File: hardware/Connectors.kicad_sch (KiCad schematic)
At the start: 18 parts, among them J1 USB_C_Receptacle_USB2.0, J14 Conn_01x05, J2 M80-5302642, J3 M300-MV31045M1, J4 M80-5L10442MC, J5 M80-5L10442MC, J6 M80-5L10442MC

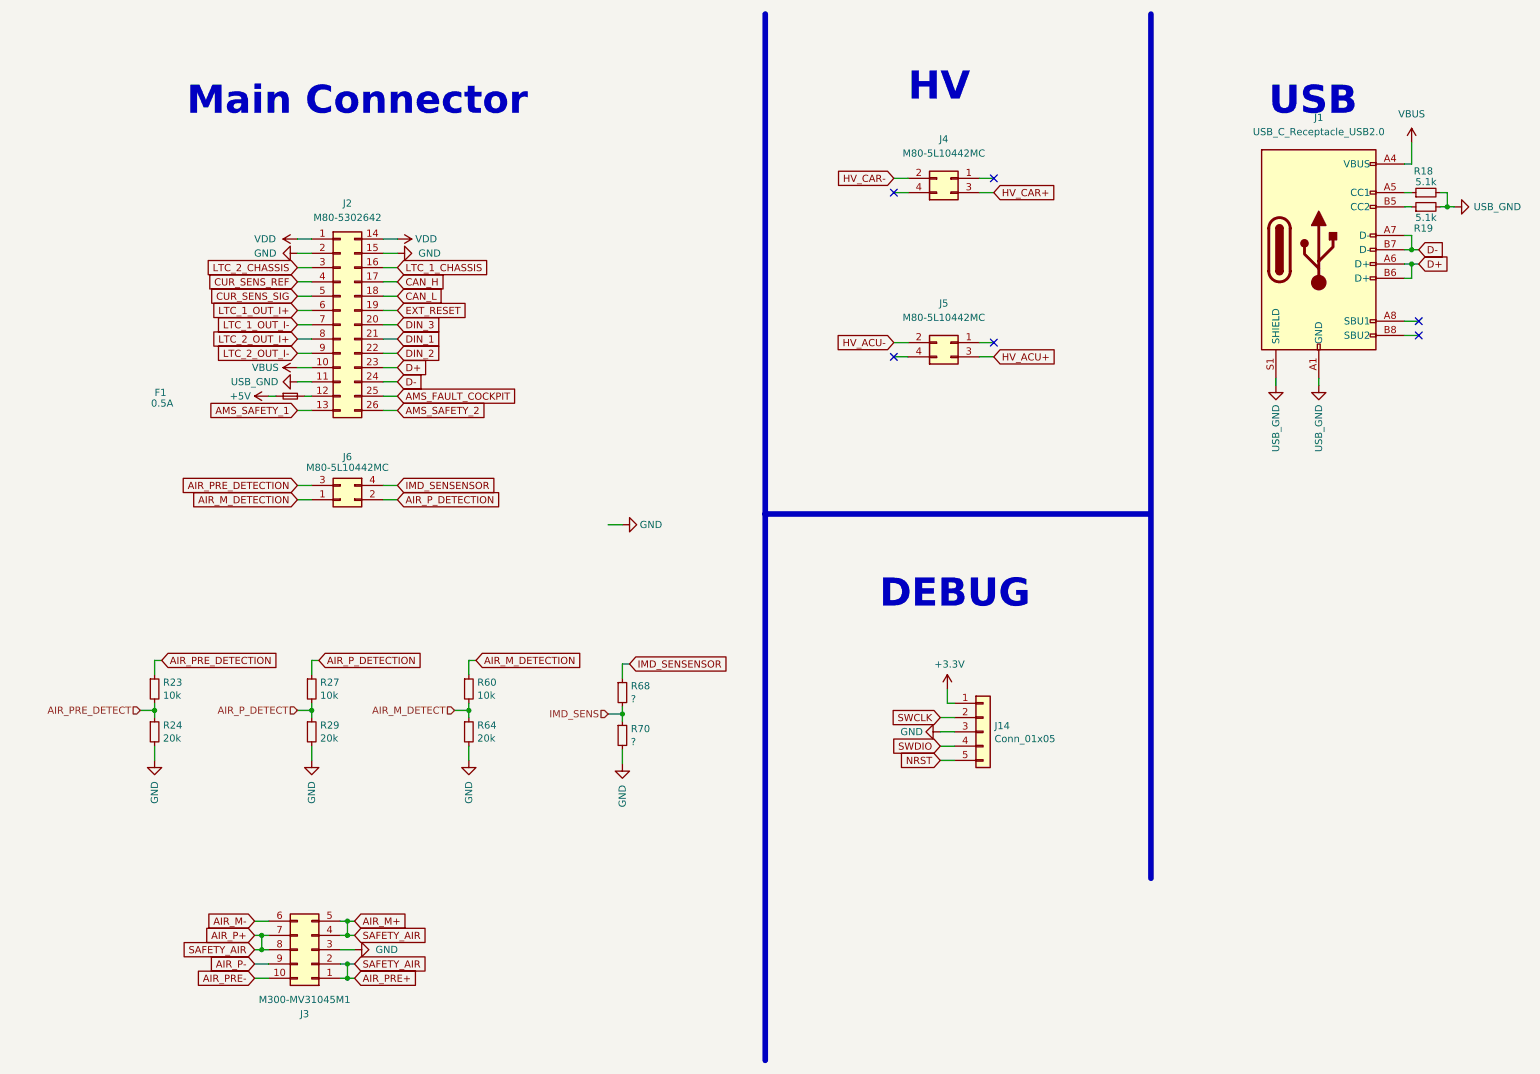
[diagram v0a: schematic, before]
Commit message: remake in progress
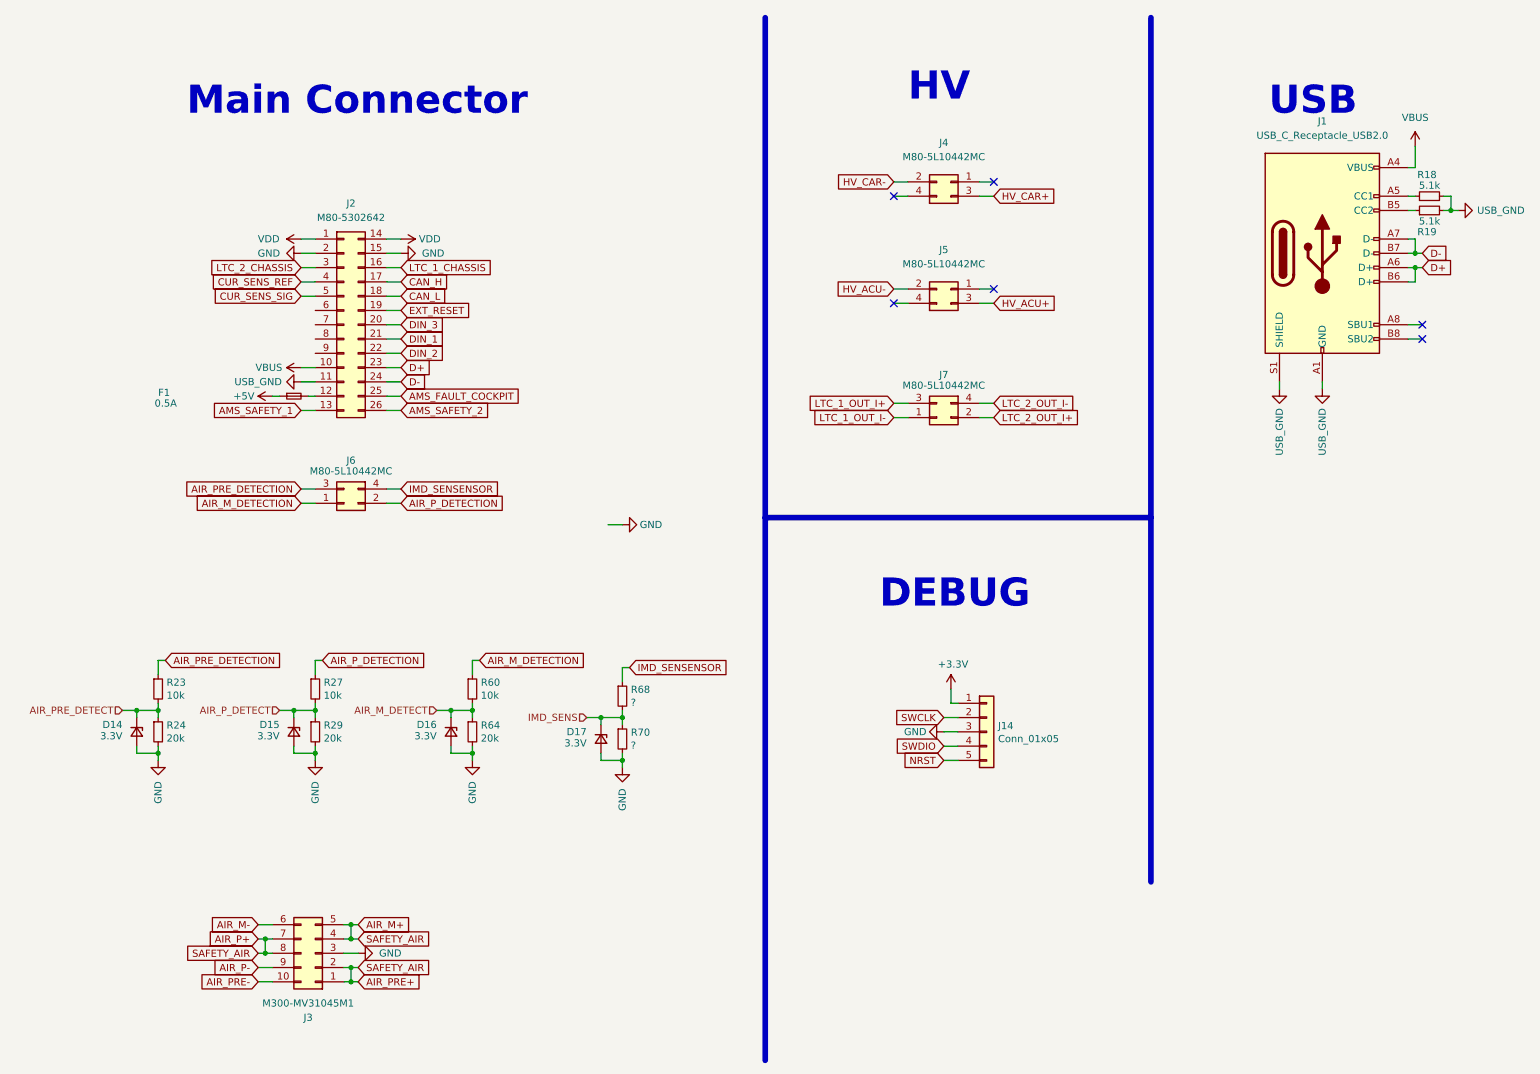
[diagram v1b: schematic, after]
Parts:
- added D14, D15, D16, D17: 3.3V, Diode_SMD:D_SOD-323_HandSoldering, symbol Device:D_Zener_Small
- added J7: M80-5L10442MC, M80-5L104YYMC, symbol M80-5L10442MC:M80-5L10442MC
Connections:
- net AIR_M_DETECT: now also D16.1 (K)
- net AIR_PRE_DETECT: now also D14.1 (K)
- net AIR_P_DETECT: now also D15.1 (K)
- net GND: now also D14.2 (A), D15.2 (A), D16.2 (A), D17.2 (A)
- net IMD_SENS: now also D17.1 (K)
- net LTC_1_OUT_I+: now also J7.3; no longer J2.6
- net LTC_1_OUT_I-: now also J7.1; no longer J2.7
- net LTC_2_OUT_I+: now also J7.2; no longer J2.8
- net LTC_2_OUT_I-: now also J7.4; no longer J2.9
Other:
- moved on the sheet: F1, J1, J14, J2, J3, J4, J5, J6, R18, R19, R23, R24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
